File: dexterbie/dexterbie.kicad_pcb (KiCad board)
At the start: 2 copper layers, 89.4 x 117.7 mm, 7 parts, among them J1 Conn_01x04_Pin, J2 Conn_01x08_Pin, SW1 SW_Push, SW2 SW_Push, U1 XIAO-ESP32-C3-SMD, U2 DHT11

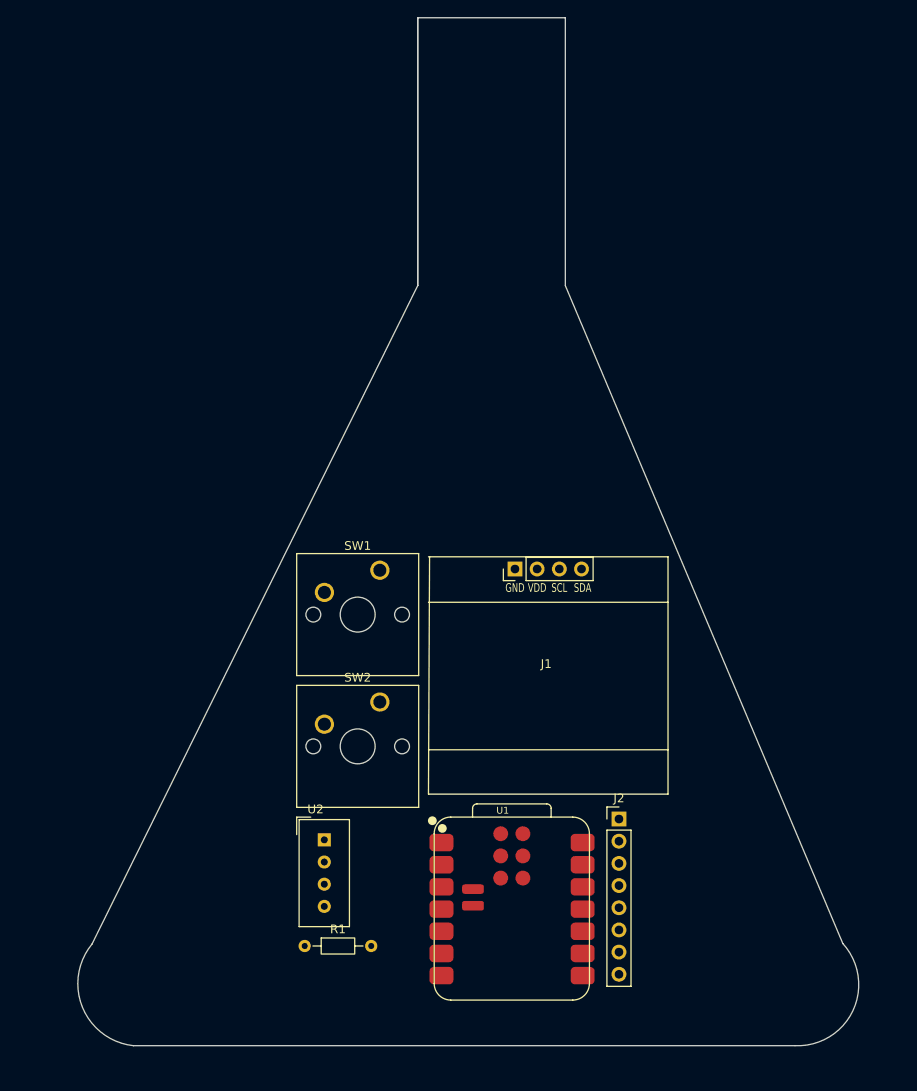
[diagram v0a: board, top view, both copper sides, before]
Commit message: feat: finish the pcb and add firmware
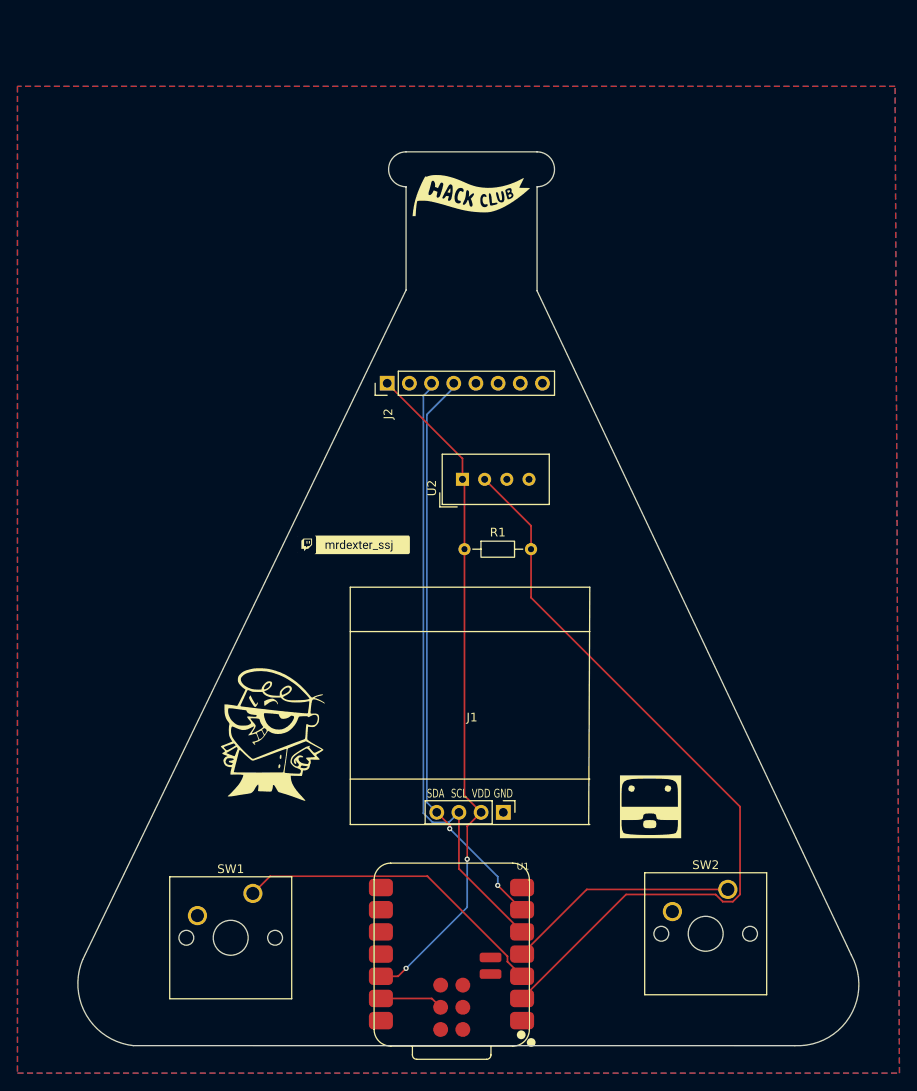
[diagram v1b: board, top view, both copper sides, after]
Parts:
- added G***: LOGO, LOGO, F.Cu at (75.0, 113.0)
- added G***: LOGO, LOGO, F.Cu at (84.5, 91.5)
- added G***: LOGO, LOGO, F.Cu at (118.5, 121.5)
- added G***: LOGO, LOGO, F.Cu at (98.0, 51.5)
- moved J2 56.5 mm to (88.3, 73.0), turned to 90 degrees
- moved R1 49.0 mm to (97.2, 92.0)
- moved SW2 45.3 mm to (127.3, 131.0)
- moved U2 44.2 mm to (97.0, 84.0), turned to 90 degrees
- moved SW1 39.8 mm to (73.0, 131.4)
- moved J1 29.3 mm to (97.8, 122.1), turned to 180 degrees
- moved U1 19.2 mm to (104.6, 127.9), turned to 180 degrees
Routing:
- net /DHT11 DATA: track 0.00 -> 90.2 mm
- net +3.3V: track 0.00 -> 78.3 mm, vias 0 -> 2
- net /SCL: track 0.00 -> 71.5 mm
- net /SDA: track 0.00 -> 66.3 mm, vias 0 -> 2
- net /GPIO2: track 0.00 -> 36.8 mm
- net /GPIO3: track 0.00 -> 26.6 mm
- net GND: track 0.00 -> 7.26 mm
- added copper zone on B.Cu, net GND
- added copper zone on F.Cu, net GND
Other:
- board size 89.4 x 117.7 mm -> 89.4 x 102.4 mm
